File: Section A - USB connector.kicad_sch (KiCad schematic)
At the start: 3 parts, among them P1 USB_C_Plug_USB2.0

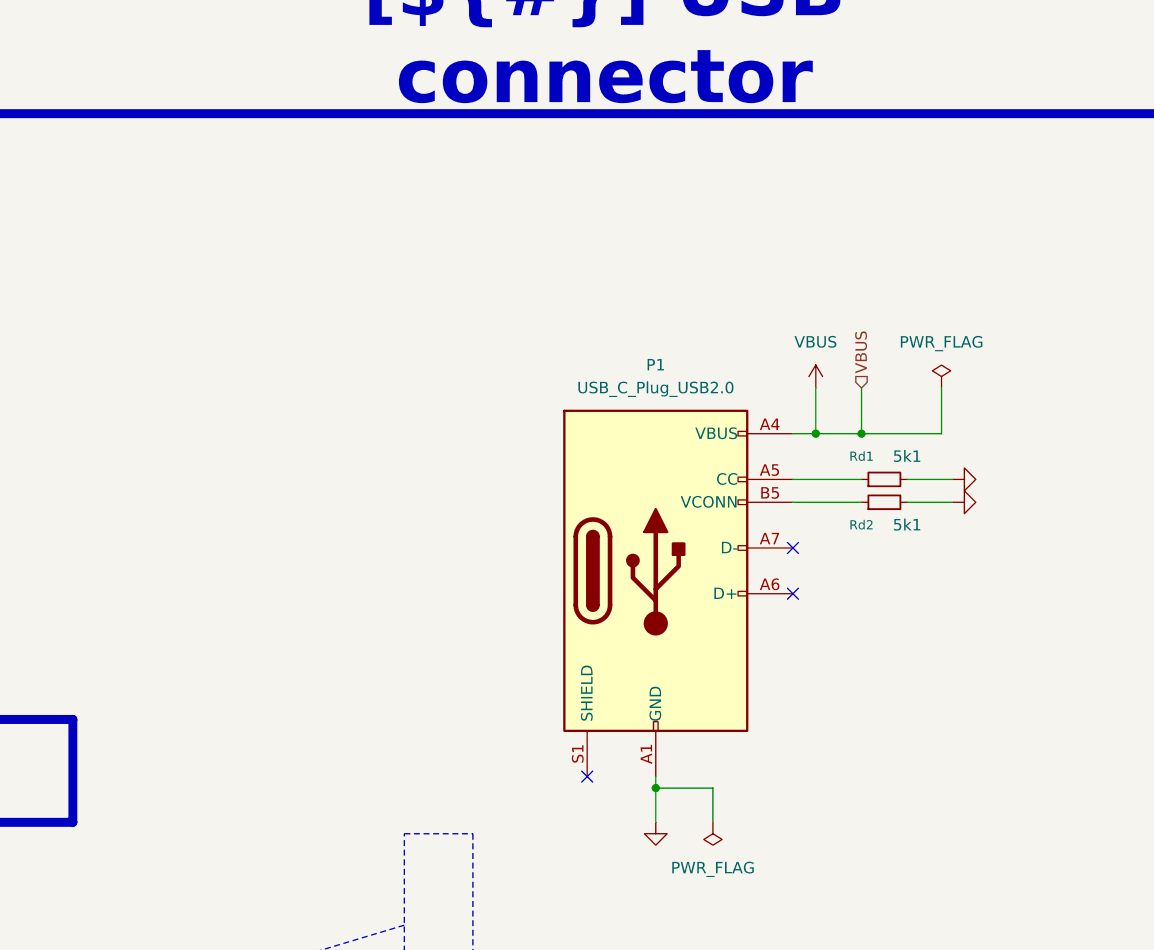
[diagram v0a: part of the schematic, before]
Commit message: pcb update
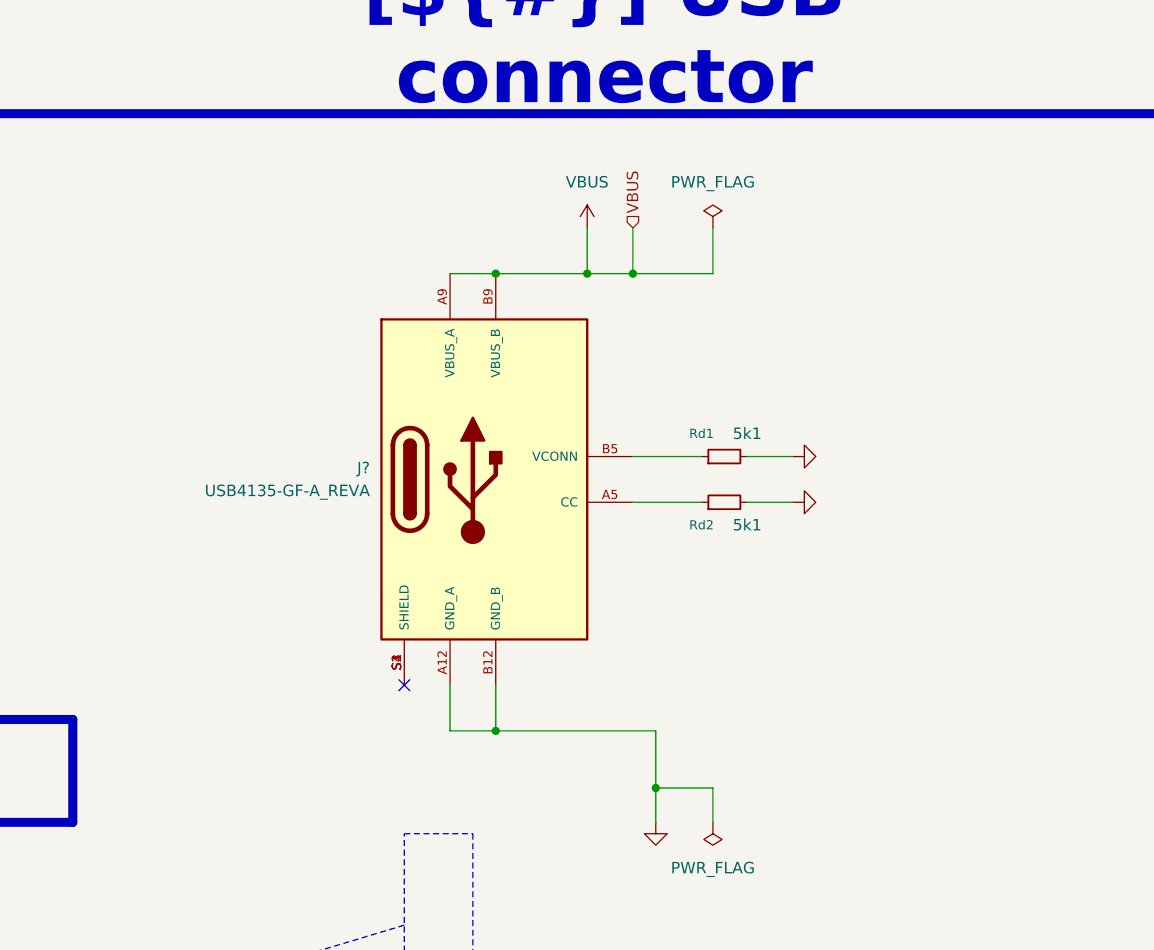
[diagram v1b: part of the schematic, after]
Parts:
- removed P1: USB_C_Plug_USB2.0, __USB4135-GF-A:GCT_USB4135-GF-A_REVA, symbol Connector:USB_C_Plug_USB2.0
- added J?: USB4135-GF-A_REVA, __USB4135-GF-A:GCT_USB4135-GF-A_REVA, symbol __GCT__USB4135-GF-A:USB4135-GF-A_REVA
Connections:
- net GND: now also J?.A12 (GND_A), J?.B12 (GND_B)
- net VBUS: now also J?.A9 (VBUS_A), J?.B9 (VBUS_B)
- net at Rd2.1: now also J?.A5 (CC)
- net at Rd1.1: now also J?.B5 (VCONN)
- new net: J?.S1 (SHIELD), J?.S2 (SHIELD), J?.S3 (SHIELD), J?.S4 (SHIELD)
- no-connect marks 3 -> 1
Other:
- moved on the sheet: Rd1, Rd2
